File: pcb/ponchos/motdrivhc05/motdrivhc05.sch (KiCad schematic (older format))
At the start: 25 parts, among them J1 MPower, J2 Screw_Terminal_1x04, J3 GW-040, J4 CONN_01X02, Q1 TIP31, Q2 TIP31, U1 L293

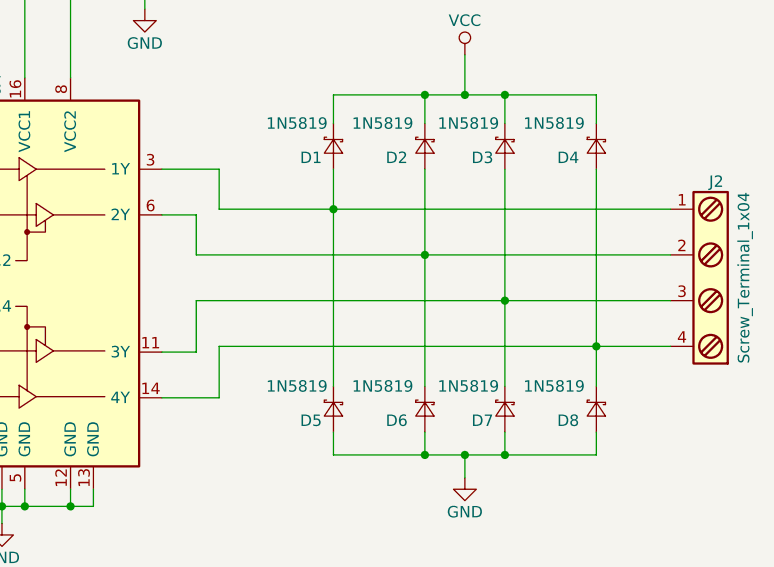
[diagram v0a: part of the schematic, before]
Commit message: Haciendo PCB...
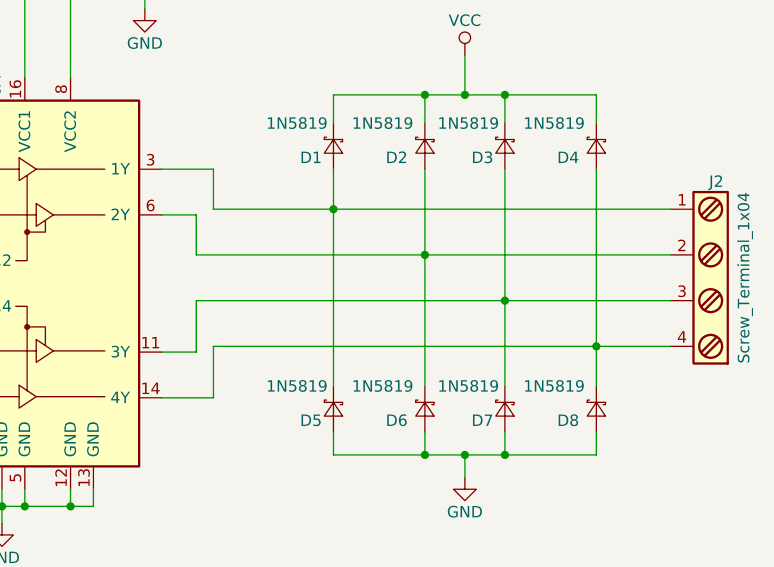
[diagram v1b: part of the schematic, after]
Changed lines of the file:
@@
 Connection ~ 7075 3675
 Wire Wire Line
-	7725 2375 9700 2375
+	7700 2375 9700 2375
 Wire Wire Line
 	7625 2575 9700 2575
@@
 	7625 2775 9700 2775
 Wire Wire Line
-	7725 2975 9700 2975
+	7700 2975 9700 2975
 Wire Wire Line
 	8225 3350 8225 3450
@@
 Wire Wire Line
 	4050 2450 4150 2450
-Wire Wire Line
-	7625 2575 7625 2400
-Wire Wire Line
-	7625 2400 7475 2400
-Wire Wire Line
-	7725 2375 7725 2200
-Wire Wire Line
-	7725 2200 7475 2200
-Wire Wire Line
-	7625 2775 7625 3000
-Wire Wire Line
-	7625 3000 7475 3000
-Wire Wire Line
-	7475 3200 7725 3200
-Wire Wire Line
-	7725 3200 7725 2975
 $Comp
 L D_Schottky_Small D7
@@
 Wire Wire Line
 	4050 4300 4275 4300
+Wire Wire Line
+	7475 2200 7700 2200
+Wire Wire Line
+	7700 2200 7700 2375
+Wire Wire Line
+	7625 2575 7625 2400
+Wire Wire Line
+	7625 2400 7475 2400
+Wire Wire Line
+	7700 2975 7700 3200
+Wire Wire Line
+	7700 3200 7475 3200
+Wire Wire Line
+	7625 2775 7625 3000
+Wire Wire Line
+	7625 3000 7475 3000
 $EndSCHEMATC
